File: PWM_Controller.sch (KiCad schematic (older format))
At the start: 58 parts, among them CN1 MAX10-FB, CN2 MAX10-FB, J1 Conn_01x02, J2 Conn_01x07, J3 Conn_01x07, J4 Conn_02x01, J5 Conn_01x03, J6 Conn_01x04, SW1 EC12PLGRSDVF, U1 DIR9001, U2 TAS5086, U3 74HCT541

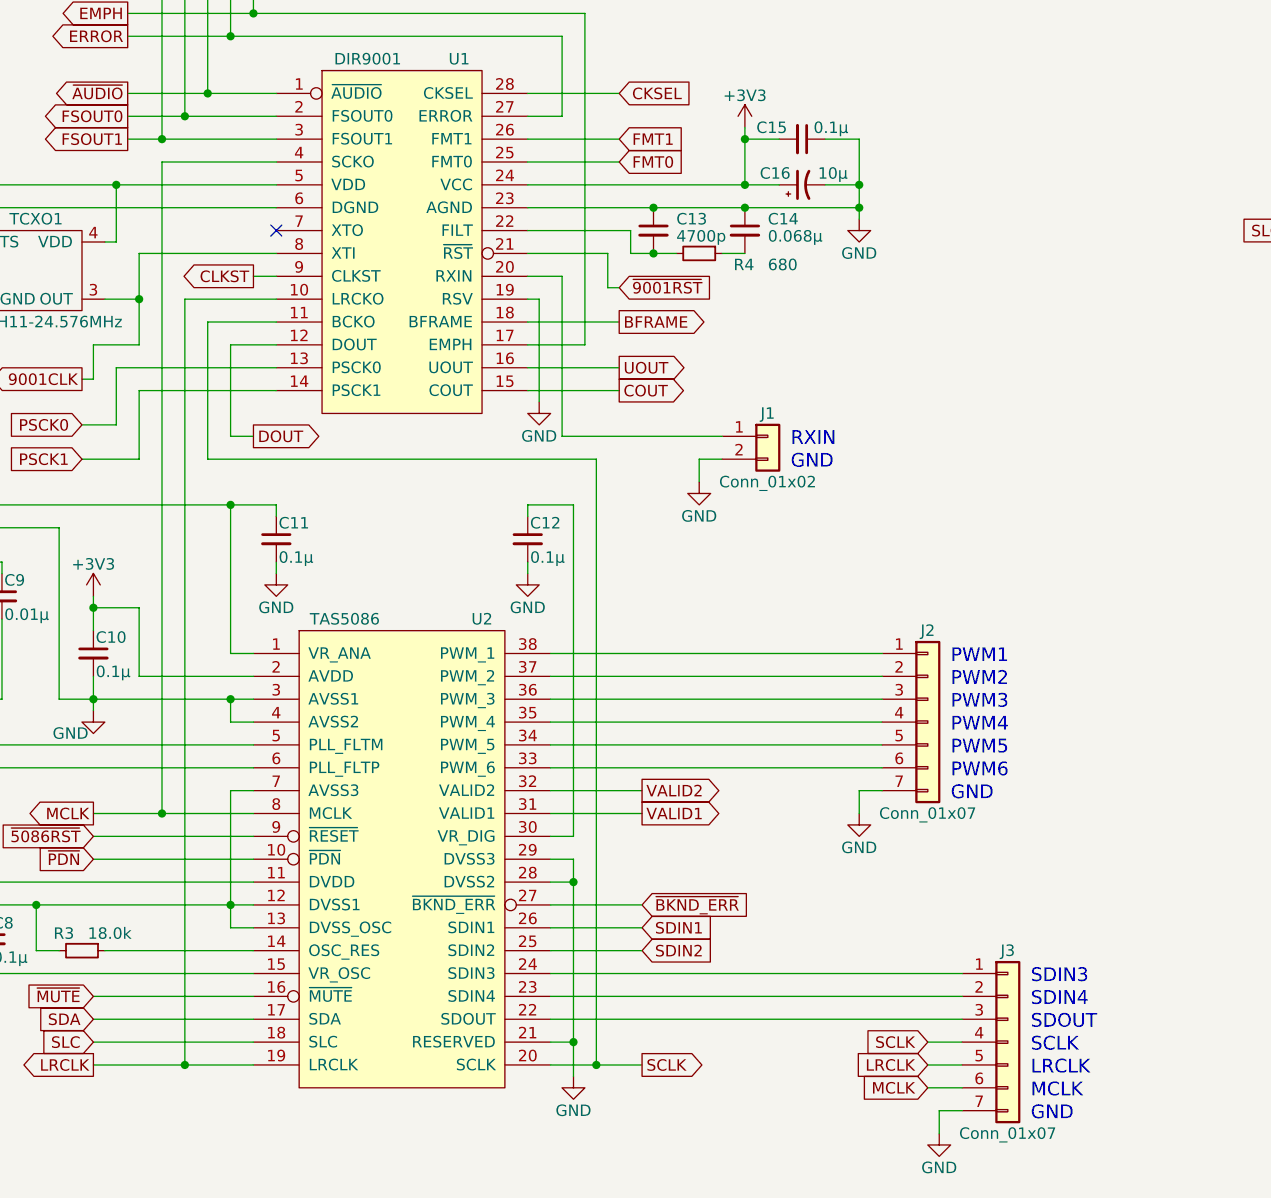
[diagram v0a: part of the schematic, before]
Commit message: Update
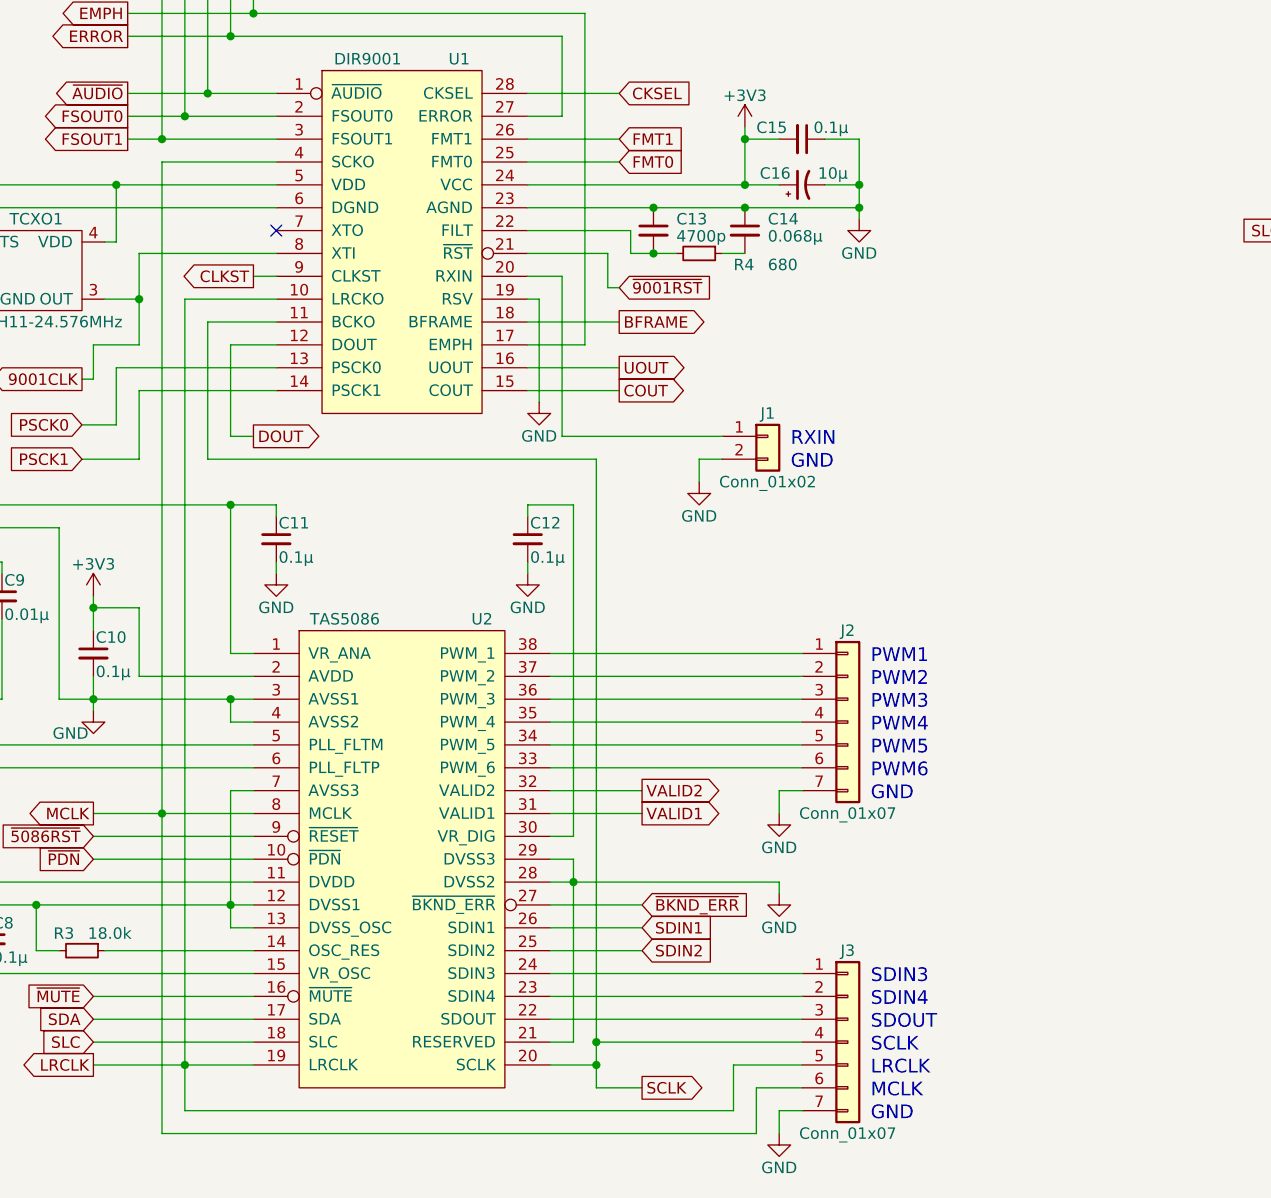
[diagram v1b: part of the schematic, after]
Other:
- moved on the sheet: J2, J3
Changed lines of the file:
@@
 L GND #PWR15
 U 1 1 5ACDBE9D
-P 4050 7350
-F 0 "#PWR15" H 4050 7100 50  0001 C CNN
-F 1 "GND" H 4050 7200 50  0000 C CNN
-F 2 "" H 4050 7350 50  0001 C CNN
-F 3 "" H 4050 7350 50  0001 C CNN
-	1    4050 7350
+P 4950 6550
+F 0 "#PWR15" H 4950 6300 50  0001 C CNN
+F 1 "GND" H 4950 6400 50  0000 C CNN
+F 2 "" H 4950 6550 50  0001 C CNN
+F 3 "" H 4950 6550 50  0001 C CNN
+	1    4950 6550
 	1    0    0    -1
 $EndComp
@@
 Text GLabel 1950 7200 0    50   Input ~ 0
 SLC
-Text GLabel 4350 7300 2    50   Output ~ 0
+Text GLabel 4350 7400 2    50   Output ~ 0
 SCLK
 Text GLabel 4350 6700 2    50   Input ~ 0
@@
 	2550 4150 2750 4150
 Wire Wire Line
-	3950 7300 4150 7300
-Wire Wire Line
-	4150 7300 4350 7300
-Wire Wire Line
 	2450 4050 2450 4650
 Wire Wire Line
@@
 	2350 7300 2650 7300
 Wire Wire Line
-	2350 7300 2350 3950
+	2350 3950 2350 7300
+Wire Wire Line
+	2350 7300 2350 7500
 Wire Wire Line
 	2350 3950 2750 3950
@@
 	4050 7200 3950 7200
 Wire Wire Line
-	4050 6400 4050 6500
-Wire Wire Line
-	4050 6500 4050 7200
-Wire Wire Line
-	4050 7200 4050 7350
-Wire Wire Line
 	3950 6400 4050 6400
-Connection ~ 4050 7200
-Wire Wire Line
-	3950 6500 4050 6500
-Connection ~ 4050 6500
 Wire Wire Line
 	3850 5150 3850 5100
@@
 	1950 7200 2650 7200
 Wire Wire Line
-	5750 6900 3950 6900
-Wire Wire Line
-	5750 7100 3950 7100
-Wire Wire Line
-	5400 5500 3950 5500
-Wire Wire Line
-	5400 5600 3950 5600
-Wire Wire Line
-	5400 5700 3950 5700
-Wire Wire Line
-	5400 5800 3950 5800
-Wire Wire Line
-	5400 5900 3950 5900
-Wire Wire Line
-	5400 6000 3950 6000
-Wire Wire Line
-	5750 7000 3950 7000
+	5050 6900 3950 6900
+Wire Wire Line
+	5050 7100 3950 7100
+Wire Wire Line
+	5050 5500 3950 5500
+Wire Wire Line
+	5050 5600 3950 5600
+Wire Wire Line
+	5050 5700 3950 5700
+Wire Wire Line
+	5050 5800 3950 5800
+Wire Wire Line
+	5050 5900 3950 5900
+Wire Wire Line
+	5050 6000 3950 6000
+Wire Wire Line
+	5050 7000 3950 7000
 Text GLabel 2650 4550 2    50   Output ~ 0
 DOUT
@@
 	2450 4650 4150 4650
 Wire Wire Line
-	4150 4650 4150 7300
-Connection ~ 4150 7300
+	4150 4650 4150 7200
+Wire Wire Line
+	4150 7200 4150 7300
+Wire Wire Line
+	4150 7300 4150 7400
 Text GLabel 1950 7300 0    50   Output ~ 0
 LRCLK
 Connection ~ 2350 7300
 Wire Wire Line
-	2250 6200 2250 3350
+	2250 3350 2250 6200
+Wire Wire Line
+	2250 6200 2250 7600
 Text GLabel 1950 6200 0    50   Output ~ 0
 MCLK
@@
 L Conn_01x07 J2
 U 1 1 5ACDBED4
-P 5600 5800
-F 0 "J2" H 5600 6200 50  0000 C CNN
-F 1 "Conn_01x07" H 5600 5400 50  0000 C CNN
-F 2 "Pin_Headers:Pin_Header_Straight_1x07_Pitch2.54mm" H 5600 5800 50  0001 C CNN
-F 3 "" H 5600 5800 50  0001 C CNN
-	1    5600 5800
+P 5250 5800
+F 0 "J2" H 5250 6200 50  0000 C CNN
+F 1 "Conn_01x07" H 5250 5400 50  0000 C CNN
+F 2 "Pin_Headers:Pin_Header_Straight_1x07_Pitch2.54mm" H 5250 5800 50  0001 C CNN
+F 3 "" H 5250 5800 50  0001 C CNN
+	1    5250 5800
 	1    0    0    -1
 $EndComp
@@
 L GND #PWR21
 U 1 1 5ACDBED5
-P 5300 6200
-F 0 "#PWR21" H 5300 5950 50  0001 C CNN
-F 1 "GND" H 5300 6050 50  0000 C CNN
-F 2 "" H 5300 6200 50  0001 C CNN
-F 3 "" H 5300 6200 50  0001 C CNN
-	1    5300 6200
-	1    0    0    -1
-$EndComp
-Wire Wire Line
-	5300 6200 5300 6100
-Wire Wire Line
-	5300 6100 5400 6100
+P 4950 6200
+F 0 "#PWR21" H 4950 5950 50  0001 C CNN
+F 1 "GND" H 4950 6050 50  0000 C CNN
+F 2 "" H 4950 6200 50  0001 C CNN
+F 3 "" H 4950 6200 50  0001 C CNN
+	1    4950 6200
+	1    0    0    -1
+$EndComp
+Wire Wire Line
+	4950 6200 4950 6100
+Wire Wire Line
+	4950 6100 5050 6100
 $Comp
 L Conn_01x07 J3
 U 1 1 5ACDBED6
-P 5950 7200
-F 0 "J3" H 5950 7600 50  0000 C CNN
-F 1 "Conn_01x07" H 5950 6800 50  0000 C CNN
-F 2 "Pin_Headers:Pin_Header_Straight_1x07_Pitch2.54mm" H 5950 7200 50  0001 C CNN
-F 3 "" H 5950 7200 50  0001 C CNN
-	1    5950 7200
+P 5250 7200
+F 0 "J3" H 5250 7600 50  0000 C CNN
+F 1 "Conn_01x07" H 5250 6800 50  0000 C CNN
+F 2 "Pin_Headers:Pin_Header_Straight_1x07_Pitch2.54mm" H 5250 7200 50  0001 C CNN
+F 3 "" H 5250 7200 50  0001 C CNN
+	1    5250 7200
 	1    0    0    -1
 $EndComp
@@
 L GND #PWR24
 U 1 1 5ACDBED7
-P 5650 7600
-F 0 "#PWR24" H 5650 7350 50  0001 C CNN
-F 1 "GND" H 5650 7450 50  0000 C CNN
-F 2 "" H 5650 7600 50  0001 C CNN
-F 3 "" H 5650 7600 50  0001 C CNN
-	1    5650 7600
-	1    0    0    -1
-$EndComp
-Text GLabel 5600 7200 0    50   Input ~ 0
-SCLK
-Text GLabel 5600 7300 0    50   Input ~ 0
-LRCLK
-Text GLabel 5600 7400 0    50   Input ~ 0
-MCLK
-Wire Wire Line
-	5600 7200 5750 7200
-Wire Wire Line
-	5750 7300 5600 7300
-Wire Wire Line
-	5750 7400 5600 7400
+P 4950 7600
+F 0 "#PWR24" H 4950 7350 50  0001 C CNN
+F 1 "GND" H 4950 7450 50  0000 C CNN
+F 2 "" H 4950 7600 50  0001 C CNN
+F 3 "" H 4950 7600 50  0001 C CNN
+	1    4950 7600
+	1    0    0    -1
+$EndComp
 $Comp
 L Conn_01x03 J5
@@
 	7550 3750 7550 3850
 Wire Wire Line
-	5650 7600 5650 7500
-Wire Wire Line
-	5650 7500 5750 7500
-Text Notes 6050 6950 0    60   ~ 0
+	4950 7600 4950 7500
+Wire Wire Line
+	4950 7500 5050 7500
+Text Notes 5350 6950 0    60   ~ 0
 SDIN3
-Text Notes 6050 7050 0    60   ~ 0
+Text Notes 5350 7050 0    60   ~ 0
 SDIN4
-Text Notes 6050 7150 0    60   ~ 0
+Text Notes 5350 7150 0    60   ~ 0
 SDOUT
-Text Notes 6050 7250 0    60   ~ 0
+Text Notes 5350 7250 0    60   ~ 0
 SCLK
-Text Notes 6050 7350 0    60   ~ 0
+Text Notes 5350 7350 0    60   ~ 0
 LRCLK
-Text Notes 6050 7450 0    60   ~ 0
+Text Notes 5350 7450 0    60   ~ 0
 MCLK
-Text Notes 6050 7550 0    60   ~ 0
+Text Notes 5350 7550 0    60   ~ 0
 GND
-Text Notes 5700 5550 0    60   ~ 0
+Text Notes 5350 5550 0    60   ~ 0
 PWM1
-Text Notes 5700 5650 0    60   ~ 0
+Text Notes 5350 5650 0    60   ~ 0
 PWM2
-Text Notes 5700 5750 0    60   ~ 0
+Text Notes 5350 5750 0    60   ~ 0
 PWM3
-Text Notes 5700 5850 0    60   ~ 0
+Text Notes 5350 5850 0    60   ~ 0
 PWM4
-Text Notes 5700 5950 0    60   ~ 0
+Text Notes 5350 5950 0    60   ~ 0
 PWM5
-Text Notes 5700 6050 0    60   ~ 0
+Text Notes 5350 6050 0    60   ~ 0
 PWM6
-Text Notes 5700 6150 0    60   ~ 0
+Text Notes 5350 6150 0    60   ~ 0
 GND
 Text Notes 5000 4600 0    60   ~ 0
@@
 	1    0    0    -1
 $EndComp
+Wire Wire Line
+	4150 7200 5050 7200
+Wire Wire Line
+	4050 6400 4050 6500
+Wire Wire Line
+	4050 6500 4050 7200
+Wire Wire Line
+	3950 6500 4050 6500
+Wire Wire Line
+	4050 6500 4950 6500
+Wire Wire Line
+	4950 6500 4950 6550
+Connection ~ 4050 6500
+Wire Wire Line
+	5050 7300 4750 7300
+Wire Wire Line
+	4750 7300 4750 7500
+Wire Wire Line
+	4750 7500 2350 7500
+Wire Wire Line
+	2250 7600 4850 7600
+Wire Wire Line
+	4850 7600 4850 7400
+Wire Wire Line
+	4850 7400 5050 7400
+Wire Wire Line
+	4150 7300 3950 7300
+Connection ~ 4150 7200
+Wire Wire Line
+	4150 7400 4350 7400
+Connection ~ 4150 7300
 $EndSCHEMATC

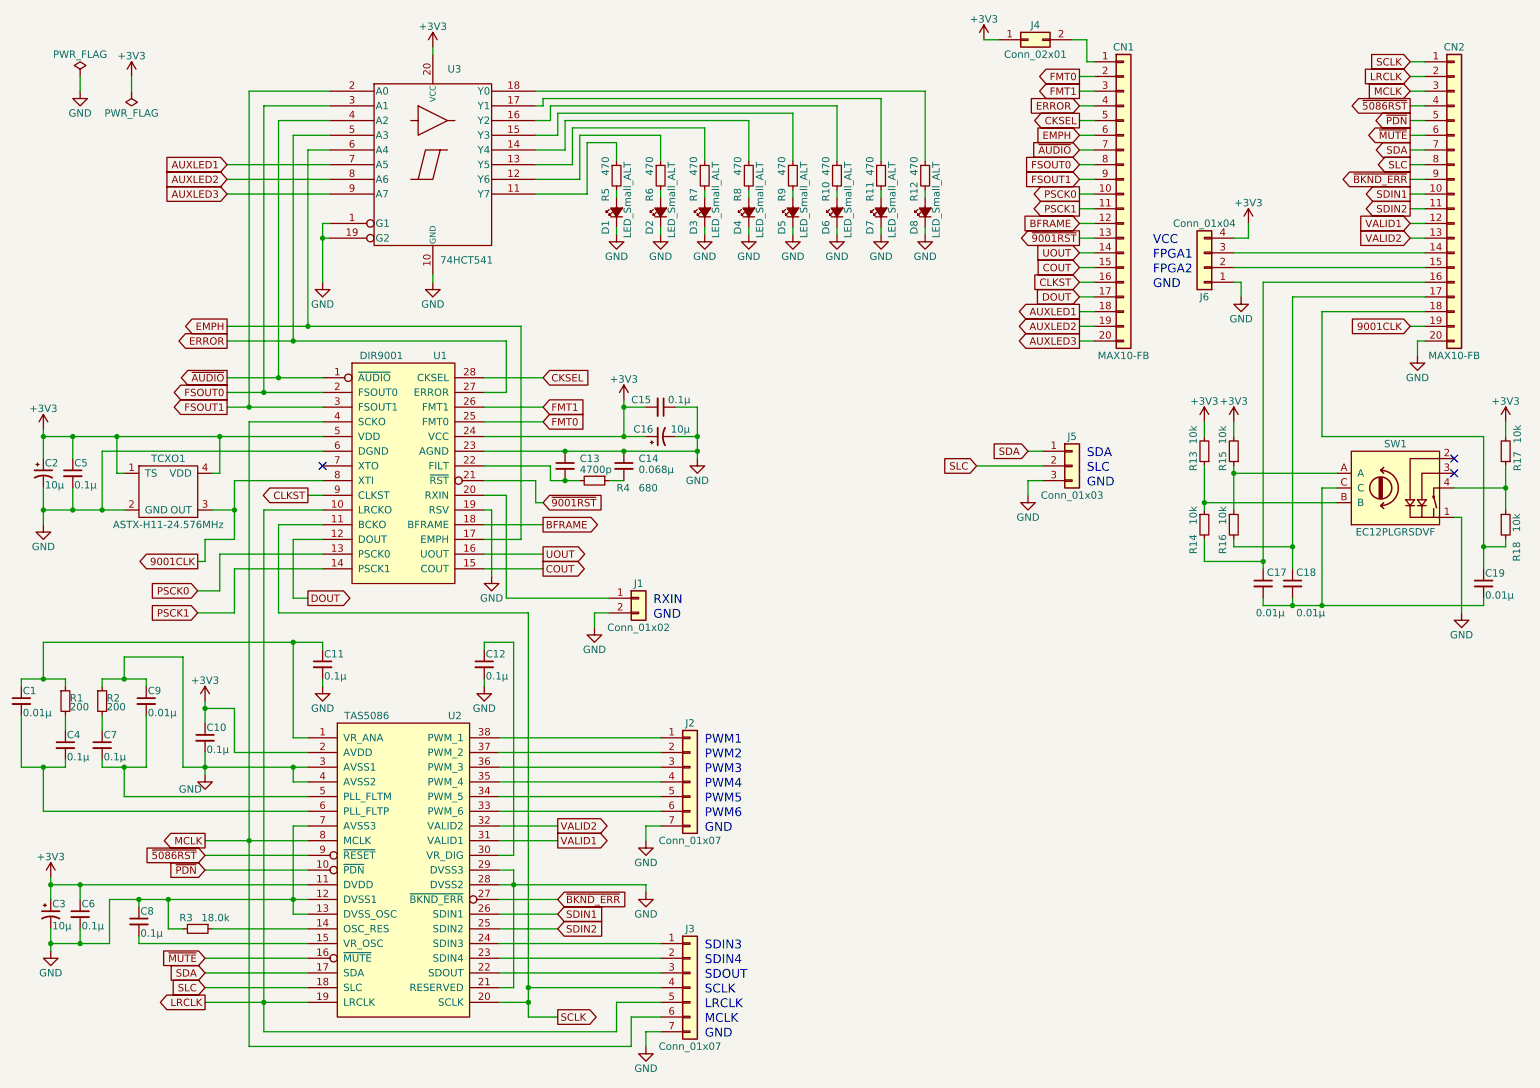
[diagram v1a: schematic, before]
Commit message: Update
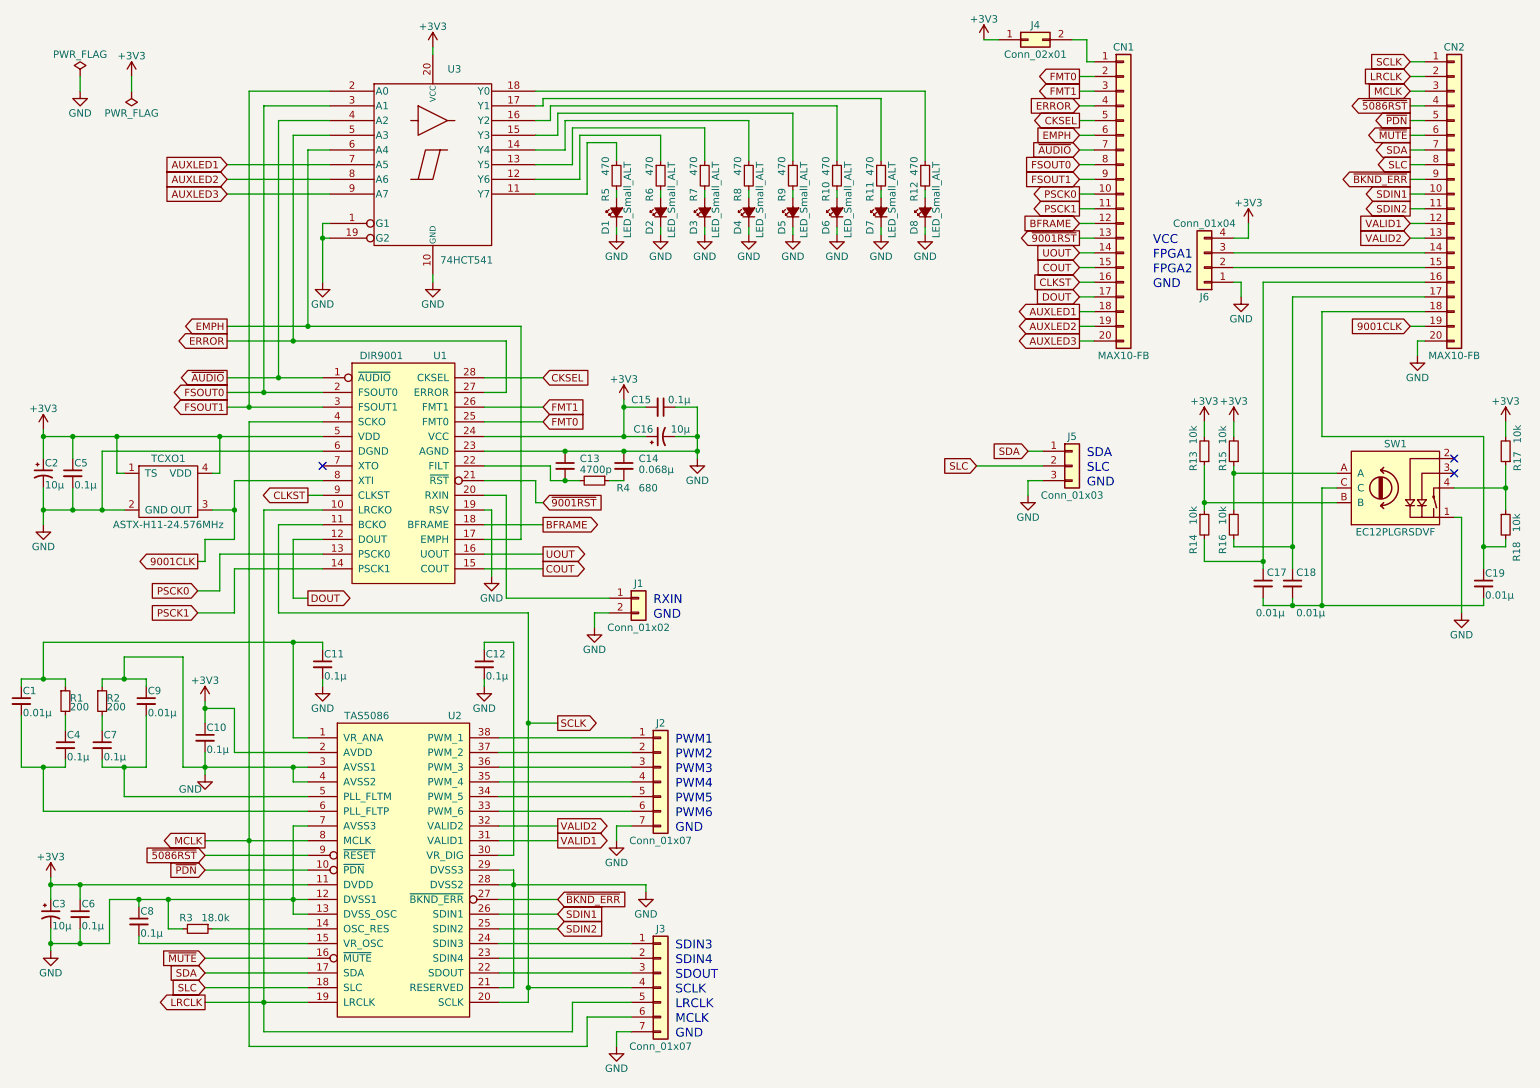
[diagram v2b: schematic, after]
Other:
- moved on the sheet: J2, J3

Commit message: KiCAD 5
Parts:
- C1, C10, C11, C12, C13, C14, C15, C17, C18, C19, C4, C5, C6, C7, C8, C9: symbol C_Small -> Device:C_Small
- C16, C2, C3: symbol CP1_Small -> Device:CP1_Small
- CN1, CN2: symbol Conn_01x20 -> PWM_Controller-rescue:Conn_01x20
- D1, D2, D3, D4, D5, D6, D7, D8: symbol LED_Small_ALT -> Device:LED_Small_ALT
- J1: symbol Conn_01x02 -> PWM_Controller-rescue:Conn_01x02
- J2, J3: symbol Conn_01x07 -> PWM_Controller-rescue:Conn_01x07
- J4: symbol Conn_02x01 -> PWM_Controller-rescue:Conn_02x01
- J5: symbol Conn_01x03 -> PWM_Controller-rescue:Conn_01x03
- J6: symbol Conn_01x04 -> PWM_Controller-rescue:Conn_01x04
- R1, R10, R11, R12, R13, R14, R15, R16, R17, R18, R2, R3, R4, R5, R6, R7, R8, R9: symbol R_Small -> Device:R_Small
- SW1: symbol EC12PLGRSDVF -> EC12P:EC12PLGRSDVF
- TCXO1: symbol ASTX-H11 -> XOSC:ASTX-H11
- U1: symbol DIR9001 -> DIR9001:DIR9001
- U2: symbol TAS5086 -> TAS5086:TAS5086
- U3: symbol 74HCT541_PWR -> PWM_Controller-rescue:74HCT541_PWR

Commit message: edit
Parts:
- SW1: symbol EC12P:EC12PLGRSDVF -> PWM_Controller-rescue:EC12PLGRSDVF-EC12P
- TCXO1: symbol XOSC:ASTX-H11 -> PWM_Controller-rescue:ASTX-H11-XOSC
- U1: symbol DIR9001:DIR9001 -> PWM_Controller-rescue:DIR9001-DIR9001
- U2: symbol TAS5086:TAS5086 -> PWM_Controller-rescue:TAS5086-TAS5086
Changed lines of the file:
@@
 	7350 750  7250 750
 $Comp
-L XOSC:ASTX-H11 TCXO1
+L PWM_Controller-rescue:ASTX-H11-XOSC TCXO1
 U 1 1 5ACDBEC1
 P 1700 3800
@@
 VCC
 $Comp
-L DIR9001:DIR9001 U1
+L PWM_Controller-rescue:DIR9001-DIR9001 U1
 U 1 1 5ACDBEDA
 P 3300 3700
@@
 $EndComp
 $Comp
-L TAS5086:TAS5086 U2
+L PWM_Controller-rescue:TAS5086-TAS5086 U2
 U 1 1 5ACDBEDB
 P 3300 6400
@@
 NoConn ~ 10450 3700
 $Comp
-L EC12P:EC12PLGRSDVF SW1
+L PWM_Controller-rescue:EC12PLGRSDVF-EC12P SW1
 U 1 1 5ACF1FB1
 P 10050 3800
